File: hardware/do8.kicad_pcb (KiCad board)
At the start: 4 copper layers, 100 x 85 mm, 116 parts, among them J101 TNG-Power-TOP, J102 TNG-Power-BTM, J103 TNG-Data-TOP, J104 TNG-Data-BTM, P102 Debug, P103 PE, P201 OUTPUT0, P202 OUTPUT1, P203 OUTPUT2, P204 OUTPUT3, Q101 FDS8449, SW101 BOOT, T101 744273222, U101 STM32F070CBT6, U102 AZ1117EH, U103 82400152, U104 TEL10, U105 TLP293, U106 STEF01, U201 ISO8200AQ, X101 8MHz

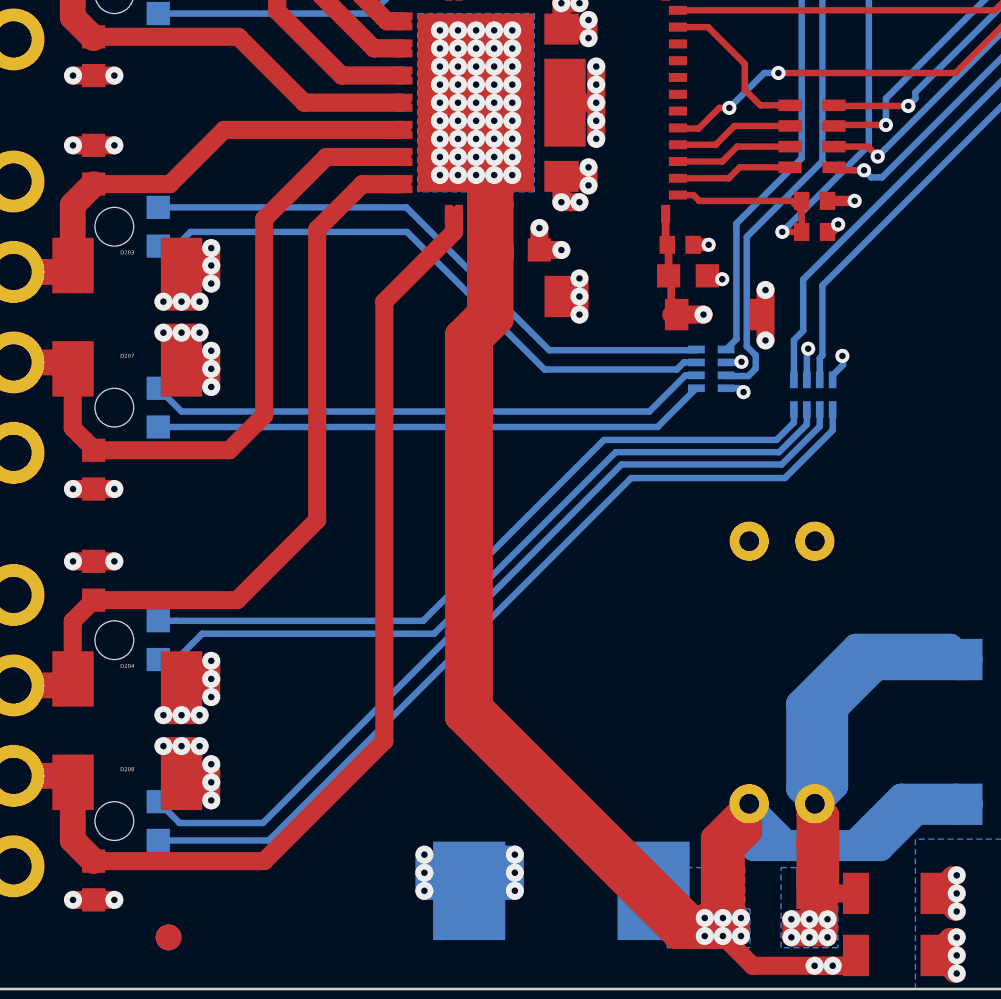
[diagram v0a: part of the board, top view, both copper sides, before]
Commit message: fix routing
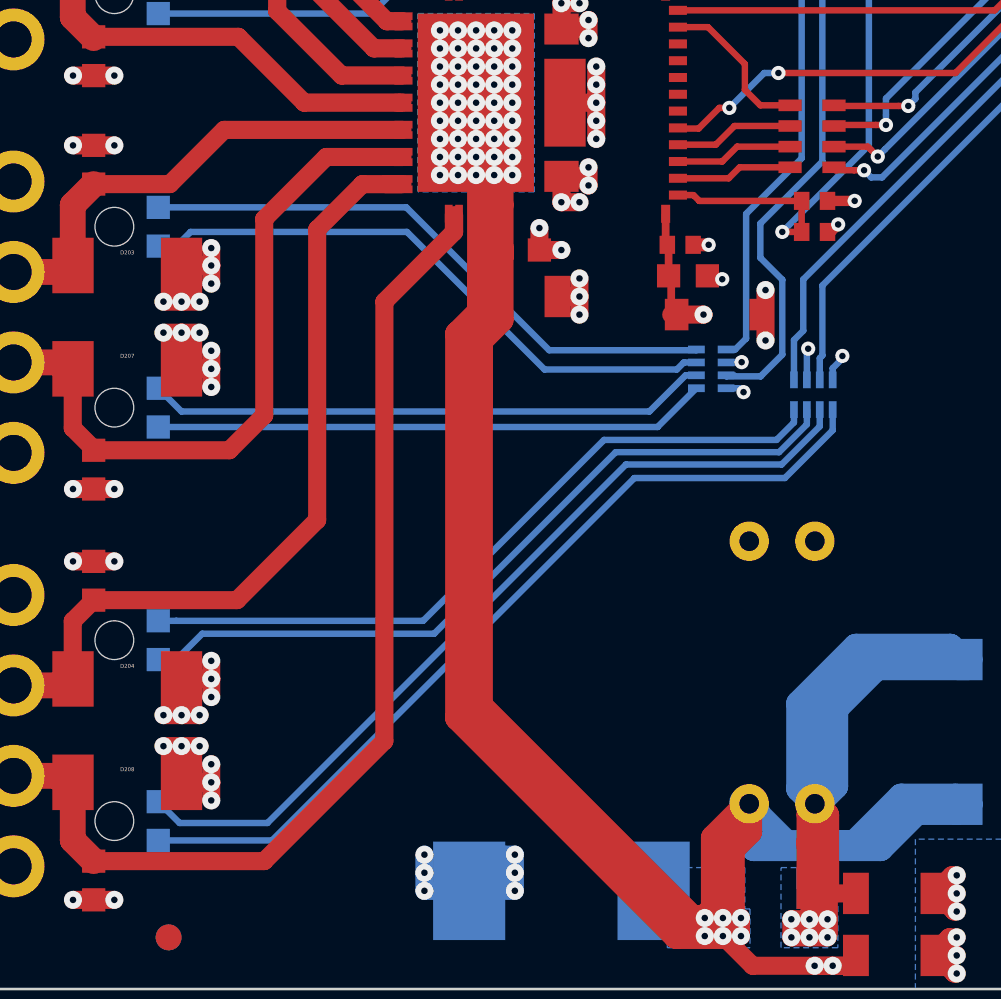
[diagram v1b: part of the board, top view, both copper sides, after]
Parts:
- C214: value 10pF -> 15pF
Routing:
- net LED5: track 70.4 -> 71.7 mm
